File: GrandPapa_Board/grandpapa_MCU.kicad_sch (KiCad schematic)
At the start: 25 parts, among them J6 Conn_02x06, U10 MCP2515-I/P, U7 MCP2562-E/SN, U8 MCP2562-E/SN, U9 PIC18F26K83, Y1 12MHz

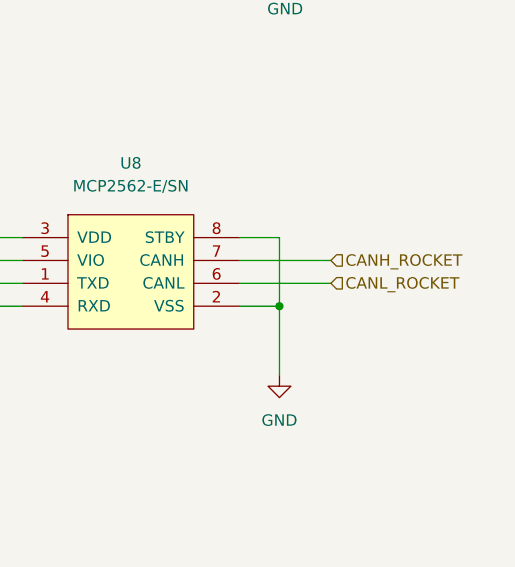
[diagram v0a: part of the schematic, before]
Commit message: update layout + routing
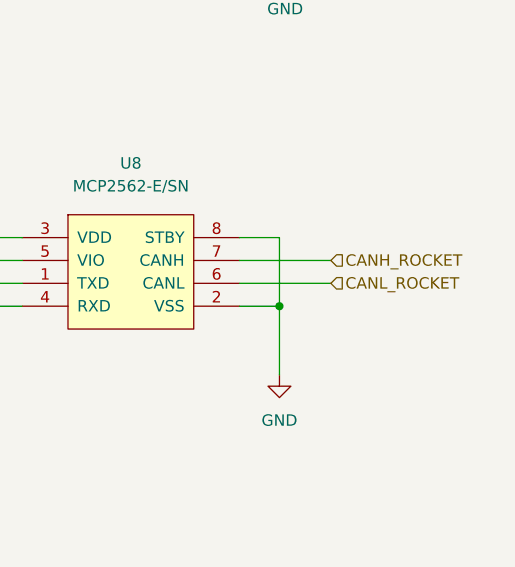
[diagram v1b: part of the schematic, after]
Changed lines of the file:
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@@
     (effects (font (size 1.27 1.27)) (justify right bottom))
-  )
-  (hierarchical_label "CANL_ROCKET" (shape input) (at 256.54 97.155 0)
-    (effects (font (size 1.27 1.27)) (justify left))
-  )
-  (hierarchical_label "CANH_ROCKET" (shape input) (at 256.54 94.615 0)
-    (effects (font (size 1.27 1.27)) (justify left))
   )
   (hierarchical_label "VBATT_VOLT_SENSE" (shape input) (at 87.63 113.03 180)
@@
   )
   (hierarchical_label "BATT_CHARGER_PG" (shape input) (at 127 118.11 0)
+    (effects (font (size 1.27 1.27)) (justify left))
+  )
+  (hierarchical_label "CANL_ROCKET" (shape input) (at 256.5367 97.155 0)
     (effects (font (size 1.27 1.27)) (justify left))
   )
@@
     (effects (font (size 1.27 1.27)) (justify right))
   )
+  (hierarchical_label "CANH_ROCKET" (shape input) (at 256.54 94.615 0)
+    (effects (font (size 1.27 1.27)) (justify left))
+  )
   (hierarchical_label "CANH_PAYLOAD" (shape input) (at 257.175 48.895 0)
